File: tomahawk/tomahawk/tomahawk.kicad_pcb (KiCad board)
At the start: 2 copper layers, 79 parts, among them SW1 SW_Push, SW10 SW_Push, SW11 SW_Push, SW12 SW_Push, SW13 SW_Push, SW14 SW_Push, SW15 SW_Push, SW16 SW_Push, SW17 SW_Push, SW18 SW_Push, SW19 SW_Push, SW2 SW_Push, SW20 SW_Push, SW21 SW_Push, SW22 SW_Push, SW23 SW_Push, SW24 SW_Push, SW25 SW_Push, SW26 SW_Push, SW27 SW_Push, SW28 SW_Push, SW29 SW_Push, SW3 SW_Push, SW30 SW_Push, SW31 SW_Push, SW32 SW_Push, SW33 SW_Push, SW34 SW_Push, SW35 SW_Push, SW36 SW_Push, SW37 SW_Push, SW38 SW_Push, SW39 SW_Push, SW4 SW_Push, SW5 SW_Push, SW6 SW_Push, SW7 SW_Push, SW8 SW_Push, SW9 SW_Push

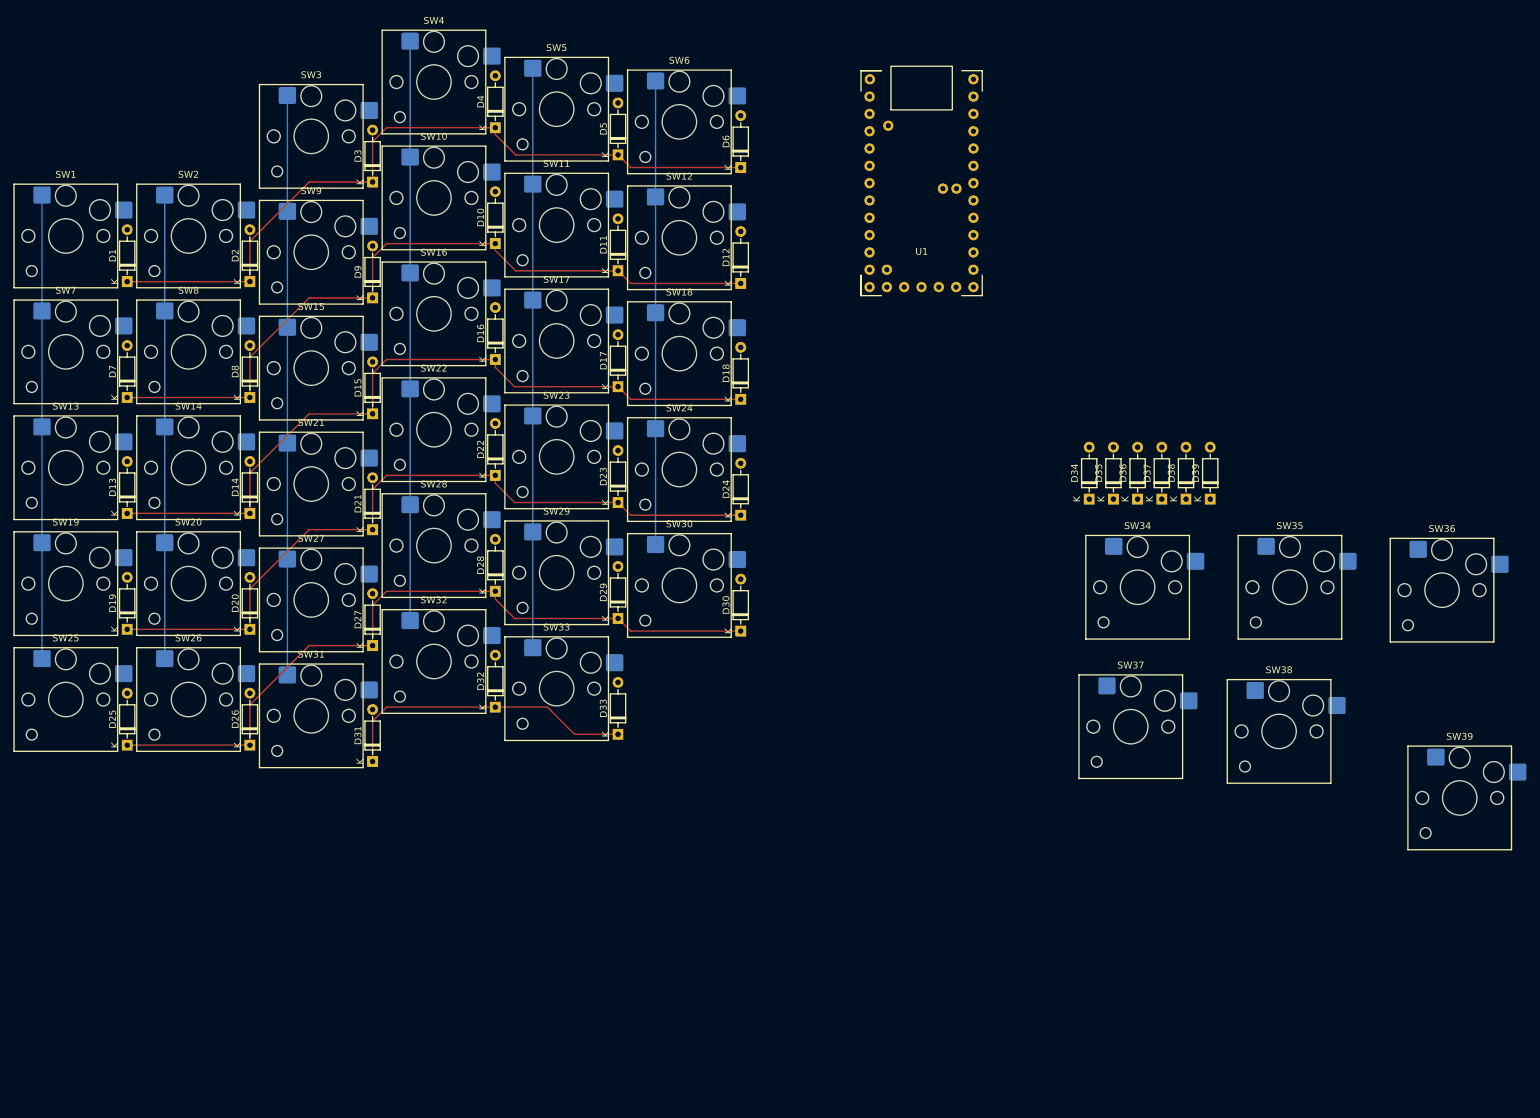
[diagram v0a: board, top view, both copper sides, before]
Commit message: wip updated diode positioning, and placed thumb cluster
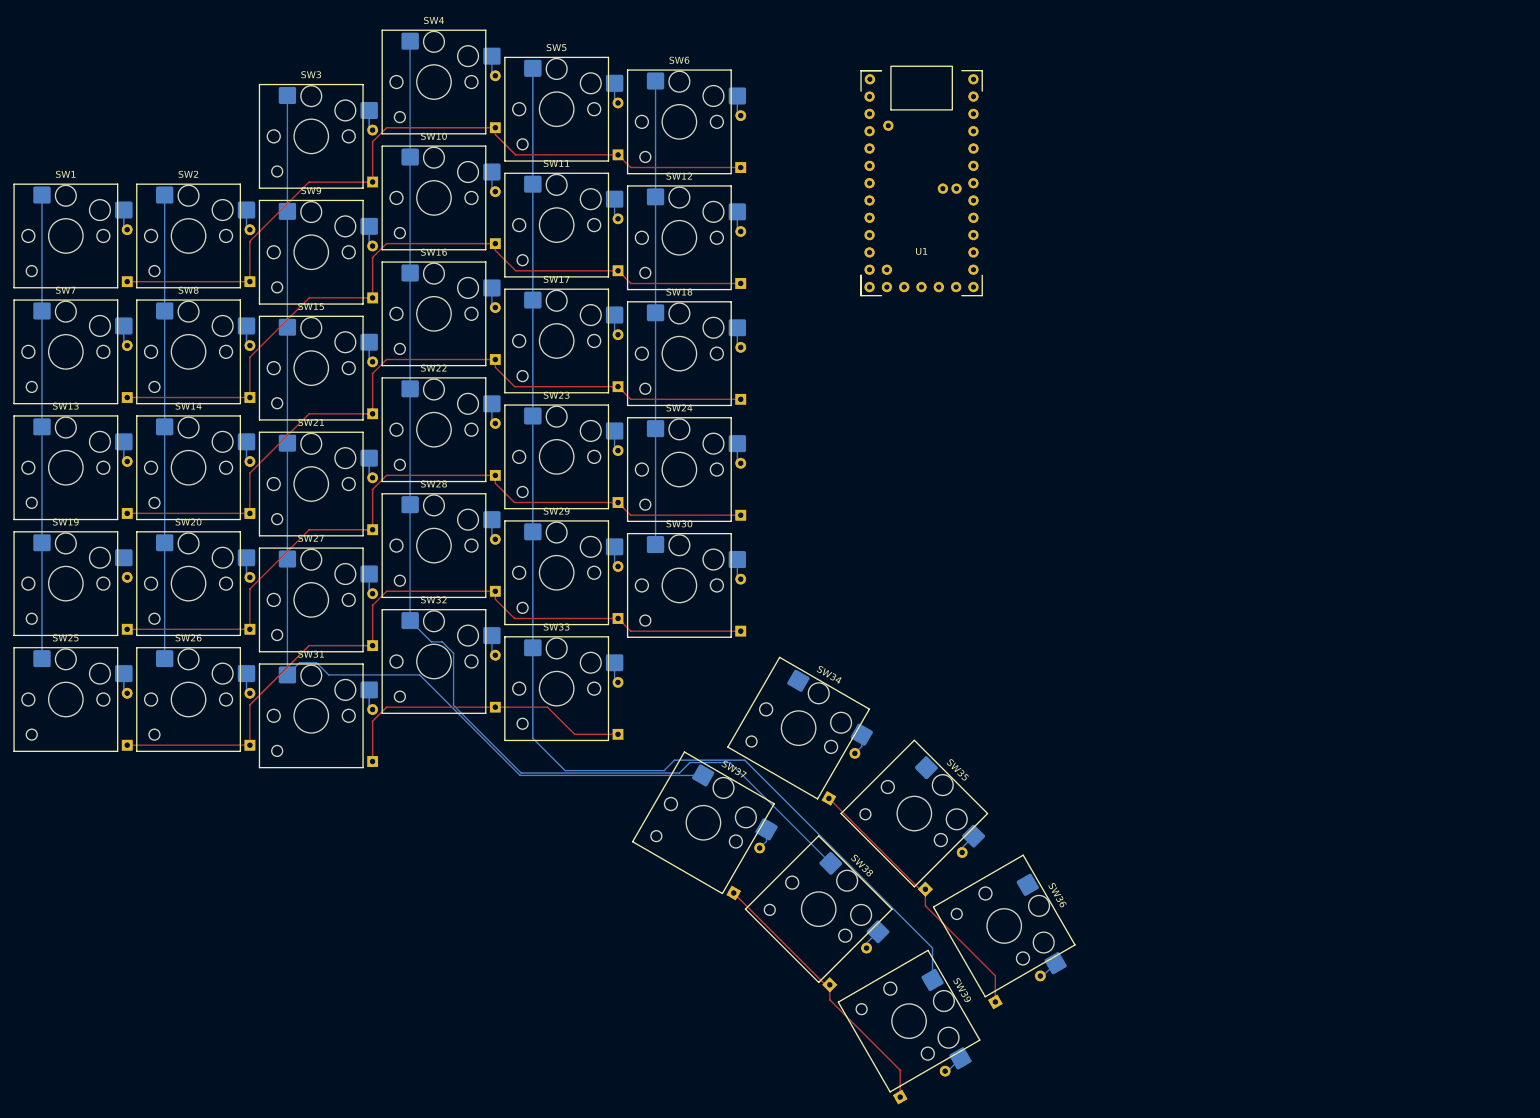
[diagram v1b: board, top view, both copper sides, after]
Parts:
- D1, D10, D11, D12, D13, D14, D15, D16, D17, D18, D19, D2, D20, D21, D22, D23, D24, D25, D26, D27, D28, D29, D3, D30, D31, D32, D33, D34, D35, D36, D37, D38, D39, D4, D5, D6, D7, D8, D9: moved to B.Cu
- moved D39 98.8 mm to (169.4, 185.8), turned to 30 degrees
- moved D38 88.4 mm to (159.1, 169.3), turned to 45 degrees
- moved SW39 87.2 mm to (170.7, 174.7), turned to -60 degrees
- moved D37 85.3 mm to (145.0, 155.9), turned to 60 degrees
- moved SW36 80.9 mm to (184.7, 160.7), turned to -60 degrees
- moved D36 76.7 mm to (183.3, 171.8), turned to 30 degrees
- moved SW38 72.4 mm to (157.4, 158.2), turned to -45 degrees
- moved SW35 64.3 mm to (171.5, 144.2), turned to -45 degrees
- moved SW37 64.3 mm to (140.5, 145.6), turned to -30 degrees
- moved D35 63.5 mm to (173.1, 155.3), turned to 45 degrees
- moved D34 58.2 mm to (158.9, 142.0), turned to 60 degrees
- moved SW34 53.9 mm to (154.5, 131.7), turned to -30 degrees
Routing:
- net COL5: track 85.0 -> 175.6 mm
- net COL4: track 85.0 -> 167.2 mm
- net COL3: track 85.0 -> 153.6 mm
- net TROW1: track 0.00 -> 40.5 mm
- net TROW2: track 0.00 -> 40.4 mm
- net Net-(D34-A): track 0.00 -> 3.16 mm
- net Net-(D37-A): track 0.00 -> 3.16 mm
- net Net-(D31-A): track 0.00 -> 3.09 mm
- net Net-(D9-A): track 0.00 -> 3.09 mm
- net Net-(D8-A): track 0.00 -> 3.09 mm
- net Net-(D7-A): track 0.00 -> 3.09 mm
- net Net-(D6-A): track 0.00 -> 3.09 mm
- net Net-(D5-A): track 0.00 -> 3.09 mm
- net Net-(D4-A): track 0.00 -> 3.09 mm
- net Net-(D33-A): track 0.00 -> 3.09 mm
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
